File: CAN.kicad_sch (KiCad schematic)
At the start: 34 parts, among them U7 MCP2515-xST, U8 SN65HVD230, Y1 16MHz

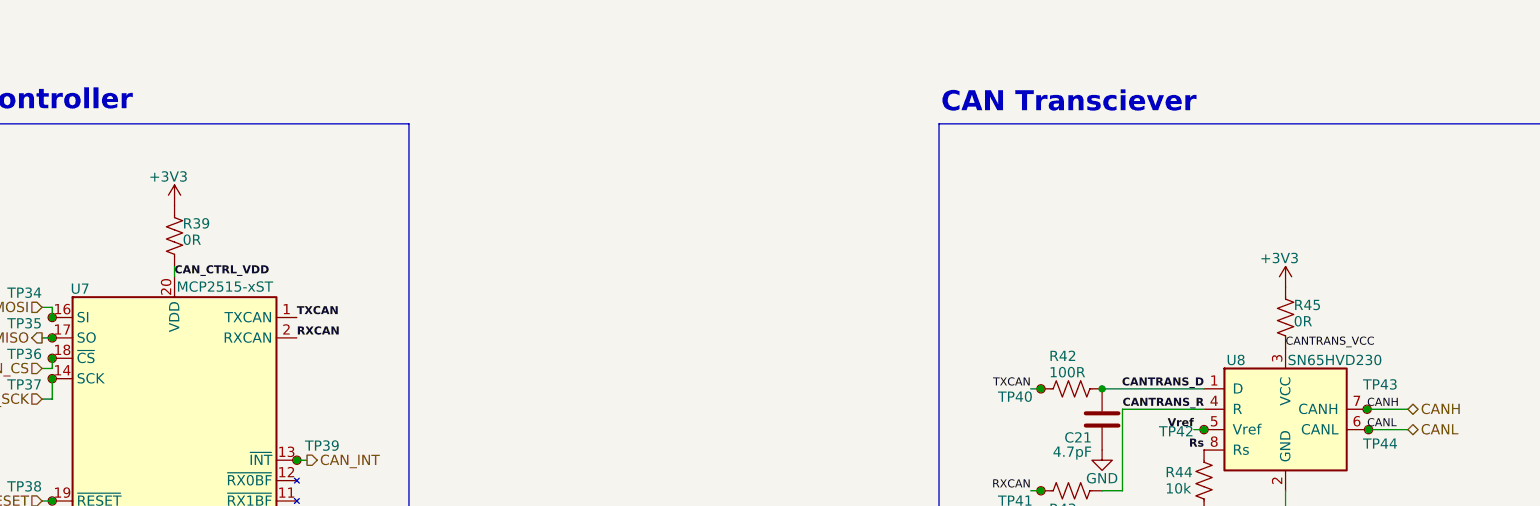
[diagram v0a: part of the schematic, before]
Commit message: Partially assigned netclasses WIP
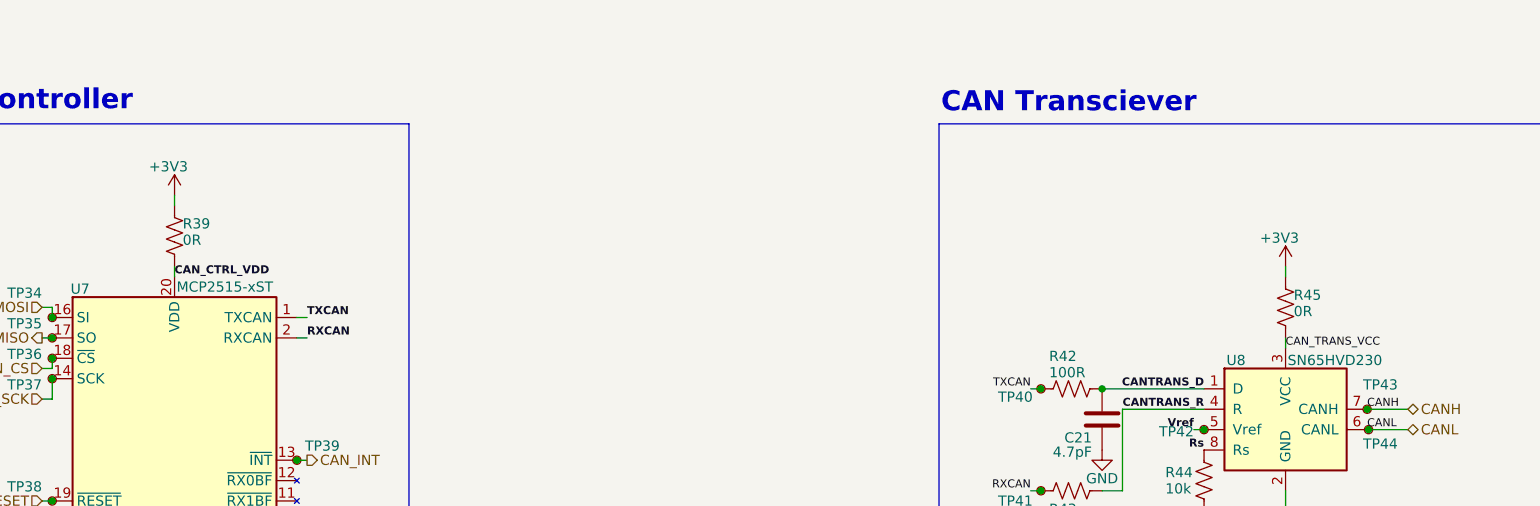
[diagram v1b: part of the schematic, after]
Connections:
- net CANTRANS_VCC renamed CAN_TRANS_VCC
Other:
- moved on the sheet: R45
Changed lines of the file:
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@@
 	(wire
 		(pts
+			(xy 69.85 57.15) (xy 69.85 58.42)
+		)
+		(stroke
+			(width 0)
+			(type default)
+		)
+	)
+	(wire
+		(pts
 			(xy 212.09 156.21) (xy 231.14 156.21)
 		)
@@
 	(wire
 		(pts
+			(xy 86.36 74.93) (xy 85.09 74.93)
+		)
+		(stroke
+			(width 0)
+			(type default)
+		)
+	)
+	(wire
+		(pts
 			(xy 53.34 143.51) (xy 50.8 143.51)
 		)
@@
 	(wire
 		(pts
+			(xy 86.36 72.39) (xy 85.09 72.39)
+		)
+		(stroke
+			(width 0)
+			(type default)
+		)
+	)
+	(wire
+		(pts
 			(xy 54.61 78.74) (xy 54.61 77.47)
 		)
@@
 	(wire
 		(pts
+			(xy 208.28 66.04) (xy 208.28 67.31)
+		)
+		(stroke
+			(width 0)
+			(type default)
+		)
+	)
+	(wire
+		(pts
 			(xy 53.34 74.93) (xy 54.61 74.93)
 		)
@@
 	(wire
 		(pts
+			(xy 208.28 74.93) (xy 208.28 76.2)
+		)
+		(stroke
+			(width 0)
+			(type default)
+		)
+	)
+	(wire
+		(pts
 			(xy 50.8 143.51) (xy 48.26 143.51)
 		)
@@
 		)
 	)
-	(label "CANTRANS_VCC"
+	(label "CAN_TRANS_VCC"
 		(at 208.28 76.2 0)
 		(effects
@@
 	)
 	(label "TXCAN"
-		(at 85.09 72.39 0)
+		(at 86.36 72.39 0)
 		(effects
 			(font
@@
 	)
 	(label "RXCAN"
-		(at 85.09 74.93 0)
+		(at 86.36 74.93 0)
 		(effects
 			(font
@@
 	(symbol
 		(lib_id "power:+3V3")
-		(at 208.28 68.58 0)
+		(at 208.28 66.04 0)
 		(unit 1)
 		(body_style 1)
@@
 		(dnp no)
 		(property "Reference" "#PWR052"
-			(at 208.28 72.39 0)
+			(at 208.28 69.85 0)
 			(hide yes)
 			(show_name no)
@@
 		)
 		(property "Value" "+3V3"
-			(at 207.518 65.024 0)
+			(at 207.518 62.484 0)
 			(show_name no)
 			(do_not_autoplace no)
@@
 		)
 		(property "Footprint" ""
-			(at 208.28 68.58 0)
+			(at 208.28 66.04 0)
 			(hide yes)
 			(show_name no)
@@
 		)
 		(property "Datasheet" ""
-			(at 208.28 68.58 0)
+			(at 208.28 66.04 0)
 			(hide yes)
 			(show_name no)
@@
 		)
 		(property "Description" "Power symbol creates a global label with name \"+3V3\""
-			(at 208.28 68.58 0)
+			(at 208.28 66.04 0)
 			(hide yes)
 			(show_name no)
@@
 	(symbol
 		(lib_id "power:+3V3")
-		(at 69.85 58.42 0)
+		(at 69.85 57.15 0)
 		(unit 1)
 		(body_style 1)
@@
 		(dnp no)
 		(property "Reference" "#PWR045"
-			(at 69.85 62.23 0)
+			(at 69.85 60.96 0)
 			(hide yes)
 			(show_name no)
@@
 		)
 		(property "Value" "+3V3"
-			(at 69.088 54.864 0)
+			(at 69.088 53.594 0)
 			(show_name no)
 			(do_not_autoplace no)
@@
 		)
 		(property "Footprint" ""
-			(at 69.85 58.42 0)
+			(at 69.85 57.15 0)
 			(hide yes)
 			(show_name no)
@@
 		)
 		(property "Datasheet" ""
-			(at 69.85 58.42 0)
+			(at 69.85 57.15 0)
 			(hide yes)
 			(show_name no)
@@
 		)
 		(property "Description" "Power symbol creates a global label with name \"+3V3\""
-			(at 69.85 58.42 0)
+			(at 69.85 57.15 0)
 			(hide yes)
 			(show_name no)
@@
 	(symbol
 		(lib_id "Device:R_US")
-		(at 208.28 72.39 0)
+		(at 208.28 71.12 0)
 		(unit 1)
 		(body_style 1)
@@
 		(dnp no)
 		(property "Reference" "R45"
-			(at 209.296 70.866 0)
+			(at 209.296 69.596 0)
 			(show_name no)
 			(do_not_autoplace no)
@@
 		)
 		(property "Value" "0R"
-			(at 209.296 72.898 0)
+			(at 209.296 71.628 0)
 			(show_name no)
 			(do_not_autoplace no)
@@
 		)
 		(property "Footprint" "Resistor_SMD:R_0805_2012Metric"
-			(at 209.296 72.644 90)
+			(at 209.296 71.374 90)
 			(hide yes)
 			(show_name no)
@@
 		)
 		(property "Datasheet" ""
-			(at 208.28 72.39 0)
+			(at 208.28 71.12 0)
 			(hide yes)
 			(show_name no)
@@
 		)
 		(property "Description" "Resistor, US symbol"
-			(at 208.28 72.39 0)
+			(at 208.28 71.12 0)
 			(hide yes)
 			(show_name no)
@@
 		)
 		(property "MFR#" ""
-			(at 208.28 72.39 0)
+			(at 208.28 71.12 0)
 			(hide yes)
 			(show_name no)
@@
 		)
 		(property "Package" "0805"
-			(at 208.28 72.39 0)
+			(at 208.28 71.12 0)
 			(hide yes)
 			(show_name no)
@@
 		)
 		(property "LCSC#" "C54921246"
-			(at 208.28 72.39 0)
+			(at 208.28 71.12 0)
 			(hide yes)
 			(show_name no)
